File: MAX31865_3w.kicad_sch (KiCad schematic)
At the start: 6 parts, among them J1 Screw_Terminal_01x03, U3 MAX31865xTP

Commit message: Passe les resistance 400 ohm en 1206
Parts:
- R1: footprint Resistor_SMD:R_0805_2012Metric_Pad1.20x1.40mm_HandSolder -> Resistor_SMD:R_1206_3216Metric_Pad1.30x1.75mm_HandSolder
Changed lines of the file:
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@@
       (effects (font (size 1.27 1.27)) (justify left))
     )
-    (property "Footprint" "Resistor_SMD:R_0805_2012Metric_Pad1.20x1.40mm_HandSolder" (id 2) (at 159.512 76.2 90)
+    (property "Footprint" "Resistor_SMD:R_1206_3216Metric_Pad1.30x1.75mm_HandSolder" (id 2) (at 159.512 76.2 90)
       (effects (font (size 1.27 1.27)) hide)
     )

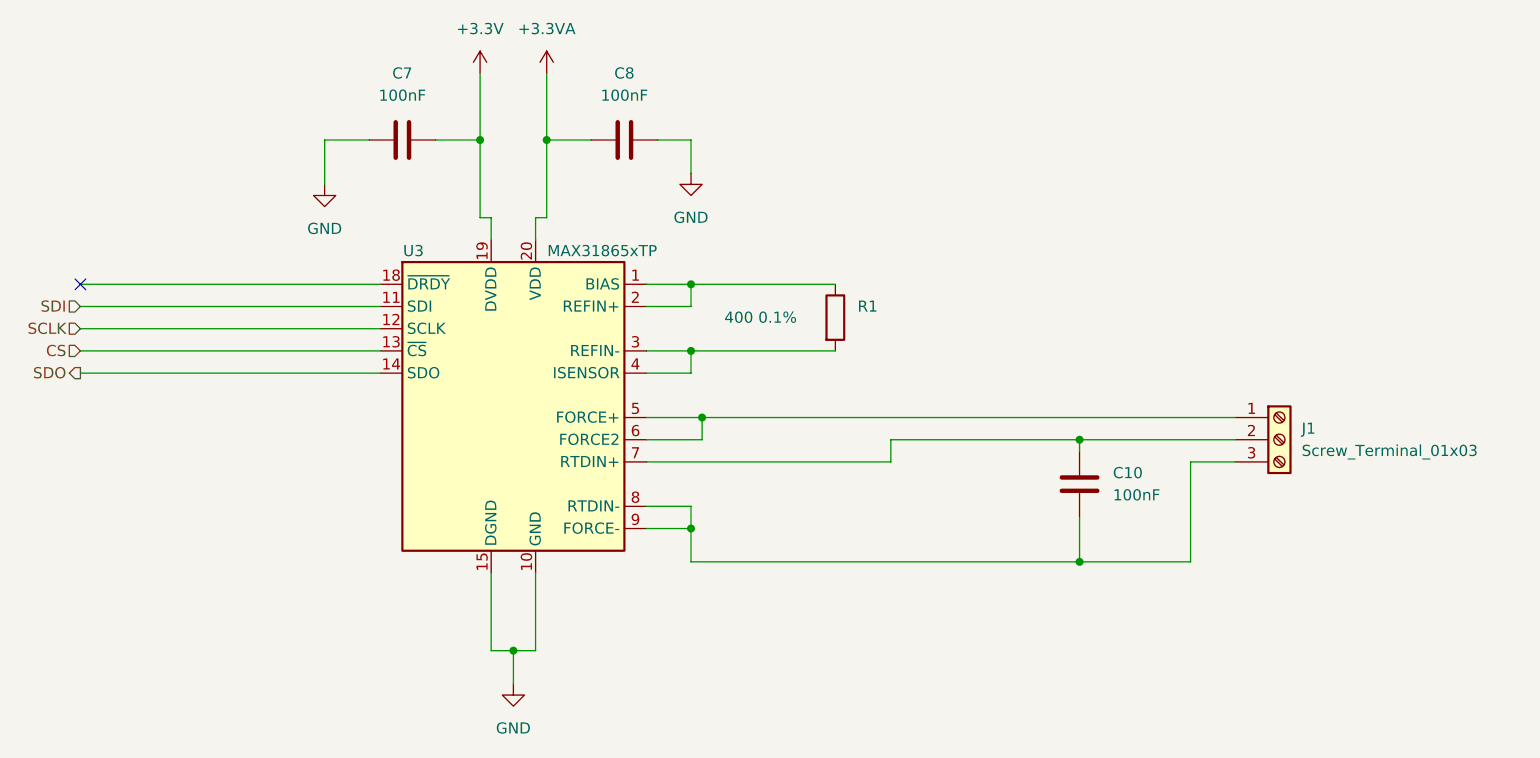
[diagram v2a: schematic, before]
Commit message: Ajoute selection 4w/3w Ajoute marquage v002
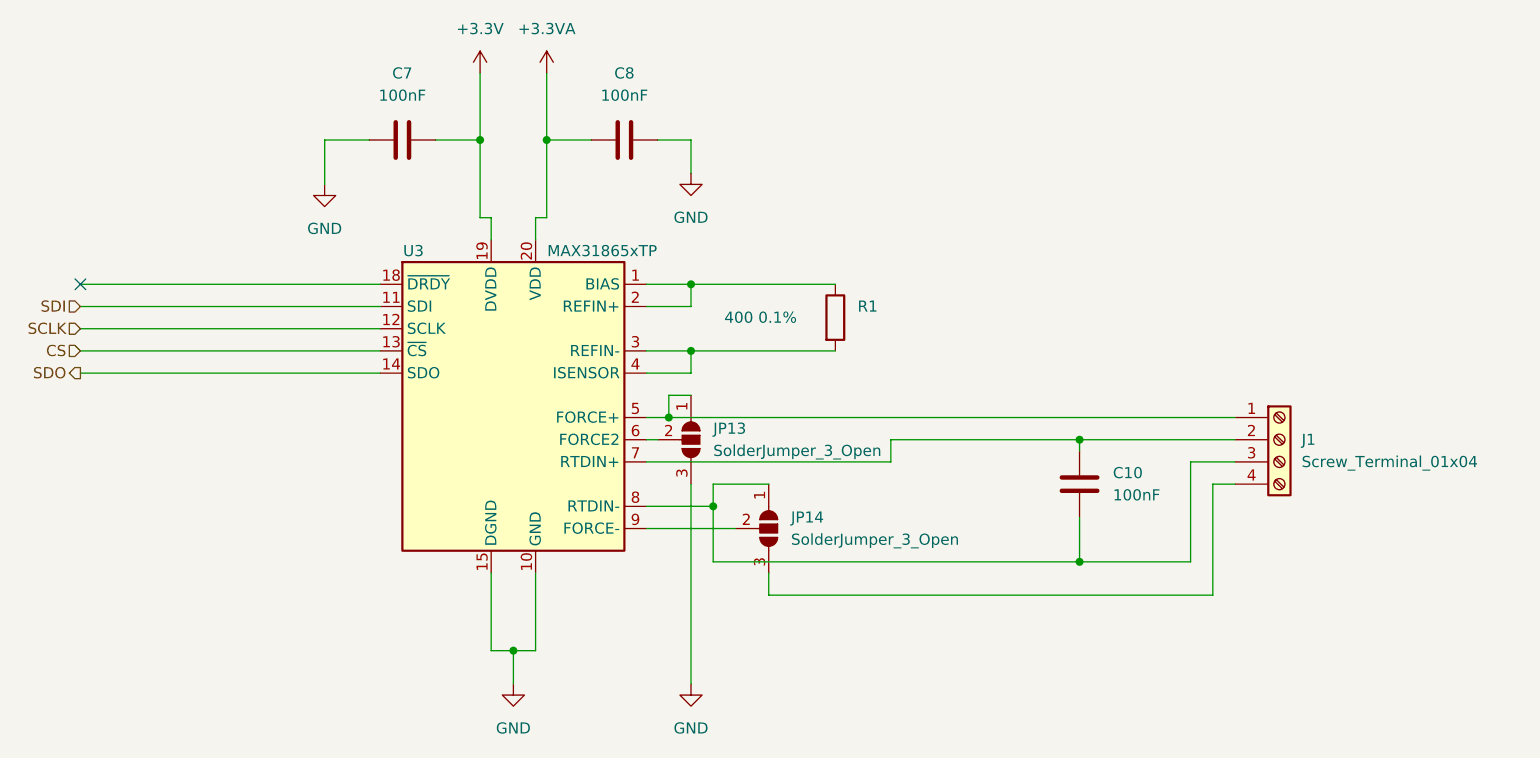
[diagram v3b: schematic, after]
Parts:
- removed J1: Screw_Terminal_01x03, TerminalBlock_Phoenix:TerminalBlock_Phoenix_MPT-0,5-3-2.54_1x03_P2.54mm_Horizontal, symbol Connector:Screw_Terminal_01x03
- added J1: Screw_Terminal_01x04, TerminalBlock_Phoenix:TerminalBlock_Phoenix_MPT-0,5-4-2.54_1x04_P2.54mm_Horizontal, symbol Connector:Screw_Terminal_01x04
- added JP13, JP14: SolderJumper_3_Open, Jumper:SolderJumper-3_P1.3mm_Open_RoundedPad1.0x1.5mm_NumberLabels, symbol Jumper:SolderJumper_3_Open
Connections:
- net GND: now also JP13.3 (B)
- net at U3.5 (FORCE+): now also J1.1 (Pin_1), JP13.1 (A); no longer U3.6 (FORCE2)
- net at C10.2, U3.7 (RTDIN+): now also J1.2 (Pin_2)
- net at C10.1, U3.8 (RTDIN-): now also J1.3 (Pin_3), JP14.1 (A); no longer U3.9 (FORCE-)
- new net: JP13.2 (C), U3.6 (FORCE2)
- new net: JP14.2 (C), U3.9 (FORCE-)
- new net: J1.4 (Pin_4), JP14.3 (B)
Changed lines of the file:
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@@
   (junction (at 144.78 72.39) (diameter 0) (color 0 0 0 0)
   )
+  (junction (at 189.23 104.14) (diameter 0) (color 0 0 0 0)
+  )
   (junction (at 144.78 80.01) (diameter 0) (color 0 0 0 0)
   )
-  (junction (at 189.23 104.14) (diameter 0) (color 0 0 0 0)
+  (junction (at 142.24 87.63) (diameter 0) (color 0 0 0 0)
   )
   (junction (at 124.46 114.3) (diameter 0) (color 0 0 0 0)
   )
-  (junction (at 146.05 87.63) (diameter 0) (color 0 0 0 0)
-  )
   (junction (at 189.23 90.17) (diameter 0) (color 0 0 0 0)
   )
-  (junction (at 144.78 100.33) (diameter 0) (color 0 0 0 0)
+  (junction (at 147.32 97.79) (diameter 0) (color 0 0 0 0)
   )
   (no_connect (at 74.93 72.39))
@@
     (stroke (width 0) (type default) (color 0 0 0 0))
   )
-  (wire (pts (xy 146.05 87.63) (xy 146.05 90.17))
-    (stroke (width 0) (type default) (color 0 0 0 0))
-  )
-  (wire (pts (xy 146.05 87.63) (xy 207.01 87.63))
-    (stroke (width 0) (type default) (color 0 0 0 0))
-  )
   (wire (pts (xy 189.23 104.14) (xy 201.93 104.14))
     (stroke (width 0) (type default) (color 0 0 0 0))
   )
-  (wire (pts (xy 139.7 87.63) (xy 146.05 87.63))
+  (wire (pts (xy 147.32 95.25) (xy 147.32 97.79))
     (stroke (width 0) (type default) (color 0 0 0 0))
   )
@@
     (stroke (width 0) (type default) (color 0 0 0 0))
   )
+  (wire (pts (xy 147.32 104.14) (xy 189.23 104.14))
+    (stroke (width 0) (type default) (color 0 0 0 0))
+  )
   (wire (pts (xy 121.92 114.3) (xy 124.46 114.3))
     (stroke (width 0) (type default) (color 0 0 0 0))
@@
     (stroke (width 0) (type default) (color 0 0 0 0))
   )
+  (wire (pts (xy 139.7 100.33) (xy 149.86 100.33))
+    (stroke (width 0) (type default) (color 0 0 0 0))
+  )
+  (wire (pts (xy 144.78 85.09) (xy 142.24 85.09))
+    (stroke (width 0) (type default) (color 0 0 0 0))
+  )
   (wire (pts (xy 128.27 48.26) (xy 128.27 55.88))
     (stroke (width 0) (type default) (color 0 0 0 0))
   )
+  (wire (pts (xy 204.47 95.25) (xy 207.01 95.25))
+    (stroke (width 0) (type default) (color 0 0 0 0))
+  )
   (wire (pts (xy 167.64 92.71) (xy 167.64 90.17))
     (stroke (width 0) (type default) (color 0 0 0 0))
   )
+  (wire (pts (xy 147.32 95.25) (xy 153.67 95.25))
+    (stroke (width 0) (type default) (color 0 0 0 0))
+  )
   (wire (pts (xy 74.93 77.47) (xy 109.22 77.47))
     (stroke (width 0) (type default) (color 0 0 0 0))
@@
     (stroke (width 0) (type default) (color 0 0 0 0))
   )
-  (wire (pts (xy 139.7 90.17) (xy 146.05 90.17))
+  (wire (pts (xy 139.7 87.63) (xy 142.24 87.63))
     (stroke (width 0) (type default) (color 0 0 0 0))
   )
@@
     (stroke (width 0) (type default) (color 0 0 0 0))
   )
-  (wire (pts (xy 144.78 100.33) (xy 144.78 104.14))
+  (wire (pts (xy 142.24 85.09) (xy 142.24 87.63))
     (stroke (width 0) (type default) (color 0 0 0 0))
   )
@@
     (stroke (width 0) (type default) (color 0 0 0 0))
   )
-  (wire (pts (xy 139.7 97.79) (xy 144.78 97.79))
+  (wire (pts (xy 153.67 107.95) (xy 204.47 107.95))
+    (stroke (width 0) (type default) (color 0 0 0 0))
+  )
+  (wire (pts (xy 139.7 97.79) (xy 147.32 97.79))
     (stroke (width 0) (type default) (color 0 0 0 0))
   )
@@
     (stroke (width 0) (type default) (color 0 0 0 0))
   )
-  (wire (pts (xy 144.78 97.79) (xy 144.78 100.33))
+  (wire (pts (xy 142.24 87.63) (xy 207.01 87.63))
     (stroke (width 0) (type default) (color 0 0 0 0))
   )
@@
     (stroke (width 0) (type default) (color 0 0 0 0))
   )
-  (wire (pts (xy 139.7 100.33) (xy 144.78 100.33))
-    (stroke (width 0) (type default) (color 0 0 0 0))
-  )
   (wire (pts (xy 115.57 55.88) (xy 120.65 55.88))
     (stroke (width 0) (type default) (color 0 0 0 0))
@@
     (stroke (width 0) (type default) (color 0 0 0 0))
   )
+  (wire (pts (xy 147.32 97.79) (xy 147.32 104.14))
+    (stroke (width 0) (type default) (color 0 0 0 0))
+  )
   (wire (pts (xy 139.7 80.01) (xy 144.78 80.01))
     (stroke (width 0) (type default) (color 0 0 0 0))
   )
+  (wire (pts (xy 144.78 95.25) (xy 144.78 118.11))
+    (stroke (width 0) (type default) (color 0 0 0 0))
+  )
   (wire (pts (xy 127 64.77) (xy 128.27 64.77))
     (stroke (width 0) (type default) (color 0 0 0 0))
   )
+  (wire (pts (xy 204.47 107.95) (xy 204.47 95.25))
+    (stroke (width 0) (type default) (color 0 0 0 0))
+  )
   (wire (pts (xy 140.97 55.88) (xy 144.78 55.88))
     (stroke (width 0) (type default) (color 0 0 0 0))
@@
     (stroke (width 0) (type default) (color 0 0 0 0))
   )
-  (wire (pts (xy 144.78 104.14) (xy 189.23 104.14))
-    (stroke (width 0) (type default) (color 0 0 0 0))
-  )
   (wire (pts (xy 127 114.3) (xy 124.46 114.3))
     (stroke (width 0) (type default) (color 0 0 0 0))
@@
   )
   (wire (pts (xy 102.87 55.88) (xy 102.87 60.96))
+    (stroke (width 0) (type default) (color 0 0 0 0))
+  )
+  (wire (pts (xy 139.7 90.17) (xy 140.97 90.17))
+    (stroke (width 0) (type default) (color 0 0 0 0))
+  )
+  (wire (pts (xy 153.67 105.41) (xy 153.67 107.95))
     (stroke (width 0) (type default) (color 0 0 0 0))
   )
@@
     (pin "1")
   )
-  (symbol (lib_id "Connector:Screw_Terminal_01x03") (at 212.09 90.17 0) (unit 1)
-    (in_bom yes) (on_board yes) (fields_autoplaced)
-    (property "Reference" "J1" (id 0) (at 214.63 88.8999 0)
-      (effects (font (size 1.27 1.27)) (justify left))
-    )
-    (property "Value" "Screw_Terminal_01x03" (id 1) (at 214.63 91.4399 0)
-      (effects (font (size 1.27 1.27)) (justify left))
-    )
-    (property "Footprint" "TerminalBlock_Phoenix:TerminalBlock_Phoenix_MPT-0,5-3-2.54_1x03_P2.54mm_Horizontal" (id 2) (at 212.09 90.17 0)
-      (effects (font (size 1.27 1.27)) hide)
-    )
-    (property "Datasheet" "~" (id 3) (at 212.09 90.17 0)
+  (symbol (lib_id "Jumper:SolderJumper_3_Open") (at 144.78 90.17 270) (unit 1)
+    (in_bom yes) (on_board yes) (fields_autoplaced)
+    (property "Reference" "JP13" (id 0) (at 147.32 88.8999 90)
+      (effects (font (size 1.27 1.27)) (justify left))
+    )
+    (property "Value" "SolderJumper_3_Open" (id 1) (at 147.32 91.4399 90)
+      (effects (font (size 1.27 1.27)) (justify left))
+    )
+    (property "Footprint" "Jumper:SolderJumper-3_P1.3mm_Open_RoundedPad1.0x1.5mm_NumberLabels" (id 2) (at 144.78 90.17 0)
+      (effects (font (size 1.27 1.27)) hide)
+    )
+    (property "Datasheet" "~" (id 3) (at 144.78 90.17 0)
       (effects (font (size 1.27 1.27)) hide)
     )
@@
     )
     (property "Datasheet" "" (id 3) (at 120.65 48.26 0)
+      (effects (font (size 1.27 1.27)) hide)
+    )
+    (pin "1")
+  )
+  (symbol (lib_id "Jumper:SolderJumper_3_Open") (at 153.67 100.33 270) (unit 1)
+    (in_bom yes) (on_board yes) (fields_autoplaced)
+    (property "Reference" "JP14" (id 0) (at 156.21 99.0599 90)
+      (effects (font (size 1.27 1.27)) (justify left))
+    )
+    (property "Value" "SolderJumper_3_Open" (id 1) (at 156.21 101.5999 90)
+      (effects (font (size 1.27 1.27)) (justify left))
+    )
+    (property "Footprint" "Jumper:SolderJumper-3_P1.3mm_Open_RoundedPad1.0x1.5mm_NumberLabels" (id 2) (at 153.67 100.33 0)
+      (effects (font (size 1.27 1.27)) hide)
+    )
+    (property "Datasheet" "~" (id 3) (at 153.67 100.33 0)
+      (effects (font (size 1.27 1.27)) hide)
+    )
+    (pin "1")
+    (pin "2")
+    (pin "3")
+  )
+  (symbol (lib_name "GND_1") (lib_id "power:GND") (at 144.78 118.11 0) (unit 1)
+    (in_bom yes) (on_board yes) (fields_autoplaced)
+    (property "Reference" "#PWR036" (id 0) (at 144.78 124.46 0)
+      (effects (font (size 1.27 1.27)) hide)
+    )
+    (property "Value" "GND" (id 1) (at 144.78 123.19 0))
+    (property "Footprint" "" (id 2) (at 144.78 118.11 0)
+      (effects (font (size 1.27 1.27)) hide)
+    )
+    (property "Datasheet" "" (id 3) (at 144.78 118.11 0)
       (effects (font (size 1.27 1.27)) hide)
     )
@@
     (pin "2")
   )
+  (symbol (lib_id "Connector:Screw_Terminal_01x04") (at 212.09 90.17 0) (unit 1)
+    (in_bom yes) (on_board yes) (fields_autoplaced)
+    (property "Reference" "J1" (id 0) (at 214.63 90.1699 0)
+      (effects (font (size 1.27 1.27)) (justify left))
+    )
+    (property "Value" "Screw_Terminal_01x04" (id 1) (at 214.63 92.7099 0)
+      (effects (font (size 1.27 1.27)) (justify left))
+    )
+    (property "Footprint" "TerminalBlock_Phoenix:TerminalBlock_Phoenix_MPT-0,5-4-2.54_1x04_P2.54mm_Horizontal" (id 2) (at 212.09 90.17 0)
+      (effects (font (size 1.27 1.27)) hide)
+    )
+    (property "Datasheet" "~" (id 3) (at 212.09 90.17 0)
+      (effects (font (size 1.27 1.27)) hide)
+    )
+    (pin "1")
+    (pin "2")
+    (pin "3")
+    (pin "4")
+  )
   (symbol (lib_id "power:GND") (at 102.87 60.96 0) (unit 1)
